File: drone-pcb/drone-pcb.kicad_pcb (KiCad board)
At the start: 2 copper layers, 50 x 50 mm, 13 parts, among them Q1 NMOS, Q2 NPN, Q3 NPN, U1 XIAO ESP32C3

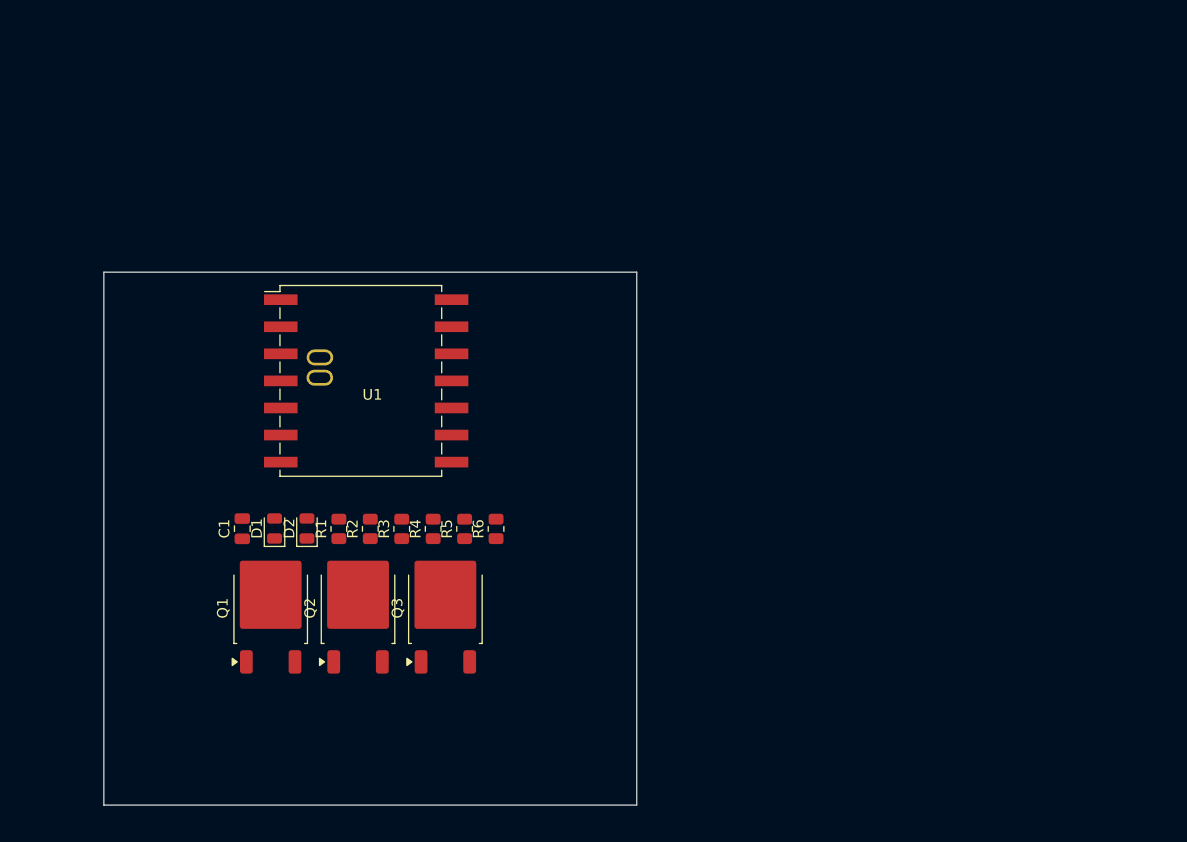
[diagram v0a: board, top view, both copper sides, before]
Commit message: draft pcb layout
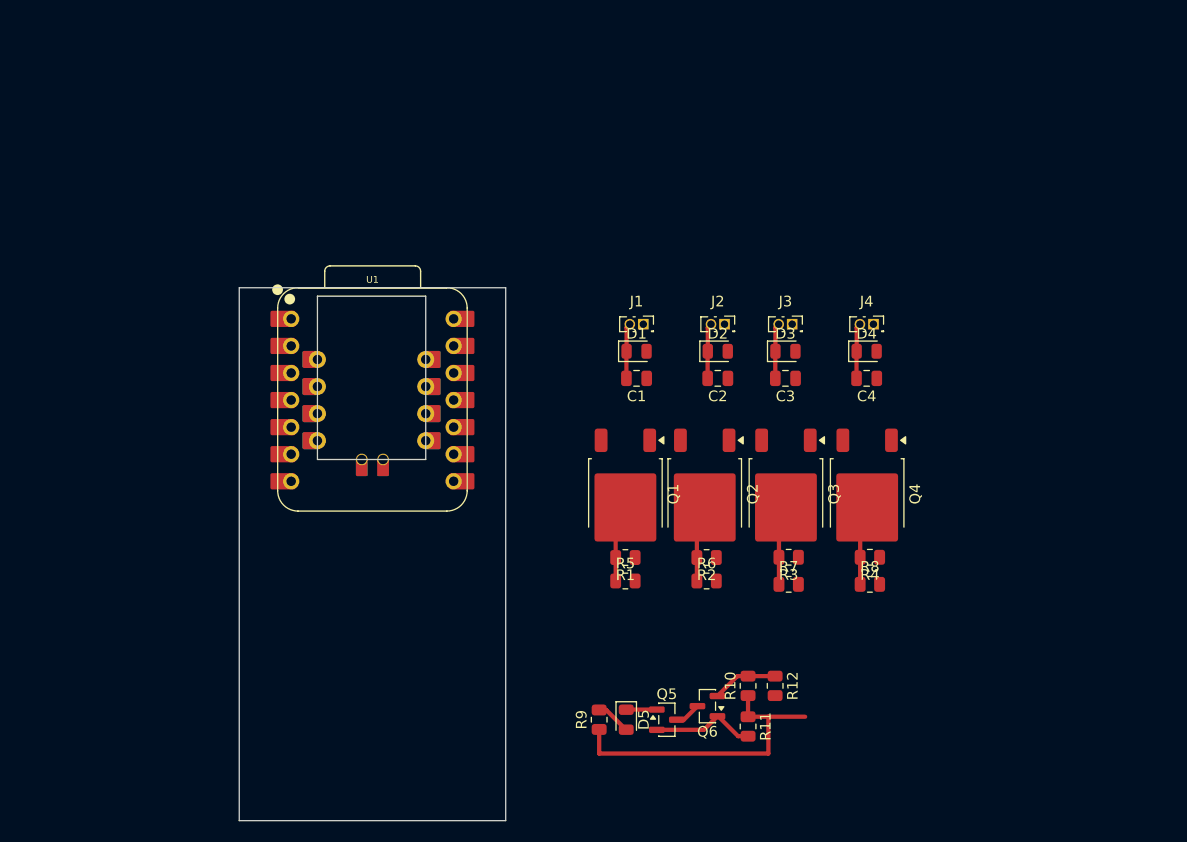
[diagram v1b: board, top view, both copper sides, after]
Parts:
- added C2: 0.1u, Capacitor_SMD:C_0805_2012Metric, F.Cu at (238.2, 48.2)
- added C3: 0.1u, Capacitor_SMD:C_0805_2012Metric, F.Cu at (244.6, 48.2)
- added C4: 0.1u, Capacitor_SMD:C_0805_2012Metric, F.Cu at (252.2, 48.2)
- added D3: 1N5819, Diode_SMD:D_0805_2012Metric, F.Cu at (244.6, 45.6)
- added D4: 1N5819, Diode_SMD:D_0805_2012Metric, F.Cu at (252.2, 45.6)
- added D5: LXZ1-PL02, Diode_SMD:D_0805_2012Metric, F.Cu at (229.6, 80.2)
- added J1: Conn_02x01, Connector_PinSocket_1.27mm:PinSocket_2x01_P1.27mm_Vertical, F.Cu at (231.2, 43.1)
- added J2: Conn_02x01, Connector_PinSocket_1.27mm:PinSocket_2x01_P1.27mm_Vertical, F.Cu at (238.8, 43.1)
- added J3: Conn_02x01, Connector_PinSocket_1.27mm:PinSocket_2x01_P1.27mm_Vertical, F.Cu at (245.2, 43.1)
- added J4: Conn_02x01, Connector_PinSocket_1.27mm:PinSocket_2x01_P1.27mm_Vertical, F.Cu at (252.8, 43.1)
- added Q4: NMOS, Package_TO_SOT_SMD:TO-252-2, F.Cu at (252.2, 59.0)
- added Q5: NPN, Package_TO_SOT_SMD:SOT-23, F.Cu at (233.4, 80.2)
- added Q6: NPN, Package_TO_SOT_SMD:SOT-23, F.Cu at (237.2, 78.9)
- added R10: 39k, Resistor_SMD:R_0805_2012Metric, F.Cu at (241.0, 77.0)
- added R11: 10k, Resistor_SMD:R_0805_2012Metric, F.Cu at (241.0, 80.8)
- added R12: 10k, Resistor_SMD:R_0805_2012Metric, F.Cu at (243.6, 77.0)
- added R7: 10k, Resistor_SMD:R_0805_2012Metric, F.Cu at (244.9, 67.5)
- added R8: 10k, Resistor_SMD:R_0805_2012Metric, F.Cu at (252.5, 67.5)
- added R9: 100, Resistor_SMD:R_0805_2012Metric, F.Cu at (227.1, 80.2)
- D2: value LXZ1-PL02 -> 1N5819
- Q2, Q3: value NPN -> NMOS
- R2, R4: value 10k -> 100
- R3: value 39k -> 100
- R6: value 100 -> 10k
- U1: value XIAO ESP32C3 -> XIAO-MG24-DIP; footprint libraries:xiao_esp32c3 -> libraries:XIAO-MG24-DIP
- moved D2 42.0 mm to (238.2, 45.6), turned to 0 degrees
- moved R4 41.1 mm to (252.5, 64.9), turned to 180 degrees
- moved C1 39.6 mm to (230.6, 48.2), turned to 180 degrees
- moved D1 37.8 mm to (230.6, 45.6), turned to 0 degrees
- moved R3 36.4 mm to (244.9, 64.9), turned to 180 degrees
- moved Q1 35.0 mm to (229.5, 59.0), turned to -90 degrees
- moved Q2 34.2 mm to (237.0, 59.0), turned to -90 degrees
- moved Q3 33.7 mm to (244.6, 59.0), turned to -90 degrees
- moved R2 31.7 mm to (237.2, 65.0), turned to 180 degrees
- moved R1 27.0 mm to (229.5, 65.0), turned to 180 degrees
- moved R6 20.4 mm to (237.2, 67.2), turned to 0 degrees
- moved R5 15.9 mm to (229.5, 67.2), turned to 0 degrees
- turned U1 to 90 degrees
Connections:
- net V_MOT+ renamed V_MOT1-
- net xiao_sense_G1 renamed Motor_1
- D2 pad 1: Net-(D2-K) -> V_BAT
- D2 pad 2: Net-(D2-A) -> V_MOT2-
- Q2 pad 1: Net-(Q2-C) -> V_MOT2-
- Q2 pad 2: Net-(Q2-B) -> Net-(Q2-G)
- Q3 pad 1: Net-(D2-K) -> V_MOT3-
- Q3 pad 2: Net-(Q2-C) -> Net-(Q3-G)
- R2 pad 1: Net-(Q1-G) -> Motor_2
- R2 pad 2: 0 -> Net-(Q2-G)
- R3 pad 1: V_BAT -> Motor_3
- R3 pad 2: Net-(Q2-B) -> Net-(Q3-G)
- R4 pad 1: Net-(Q2-B) -> Motor_4
- R4 pad 2: 0 -> Net-(Q4-G)
- R5 pad 1: V_BAT -> Net-(Q1-G)
- R5 pad 2: Net-(Q2-C) -> 0
- R6 pad 1: V_BAT -> Net-(Q2-G)
- R6 pad 2: Net-(D2-A) -> 0
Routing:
- net V_BAT: track 0.00 -> 49.8 mm
- net Net-(Q5-B): track 0.00 -> 9.89 mm
- net Net-(Q4-G): track 0.00 -> 7.87 mm
- net Net-(Q3-G): track 0.00 -> 7.87 mm
- net Net-(Q1-G): track 0.00 -> 7.81 mm
- net Net-(Q2-G): track 0.00 -> 7.64 mm
- net Net-(Q6-B): track 0.00 -> 6.19 mm
- net Net-(D5-A): track 0.00 -> 3.34 mm
- net Net-(D5-K): track 0.00 -> 2.88 mm
- net 0: track 0.00 -> 2.46 mm
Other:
- board size 50 x 50 mm -> 25 x 50 mm

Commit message: apdejt
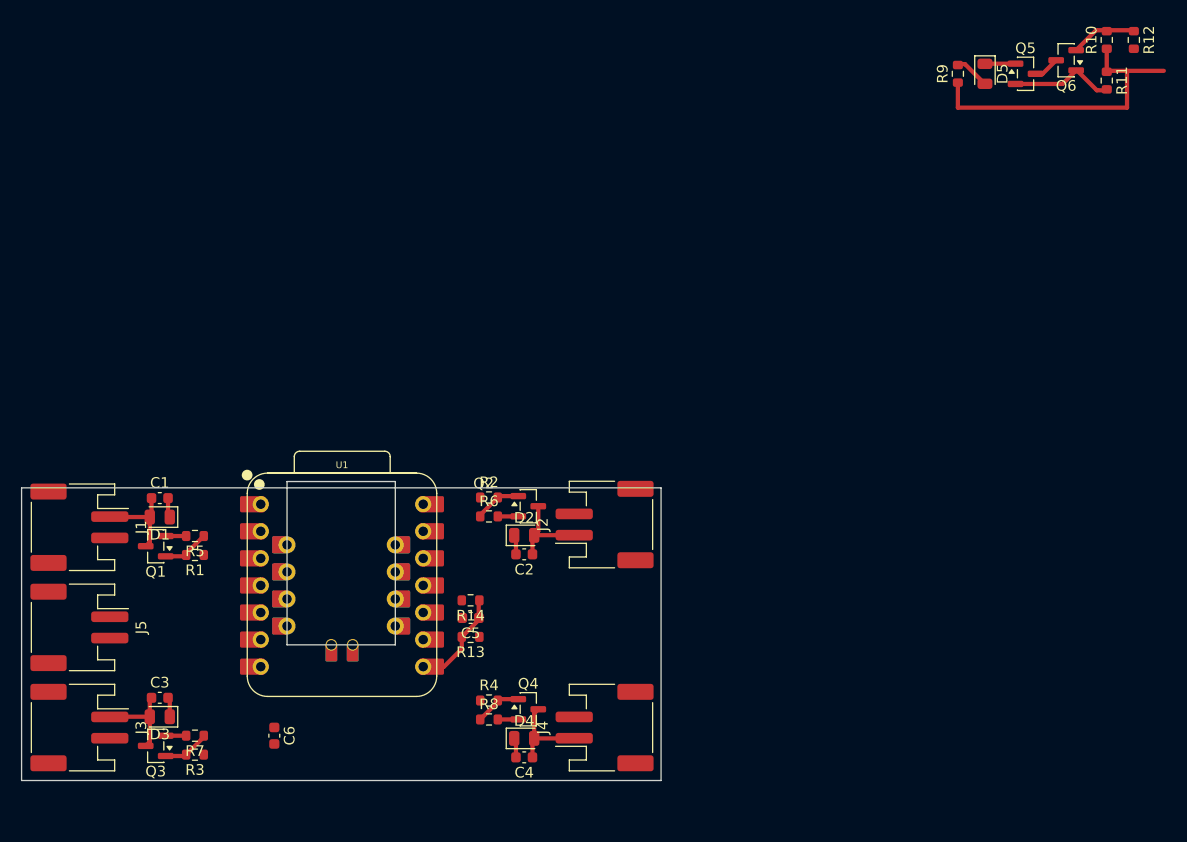
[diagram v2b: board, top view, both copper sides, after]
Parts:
- added C5: 0.1u, Capacitor_SMD:C_0603_1608Metric, F.Cu at (215.0, 70.6)
- added C6: 470u, Capacitor_SMD:C_0603_1608Metric, F.Cu at (196.6, 81.7)
- added J5: Conn_02x01, jst:JST_PH_S2B-PH-SM4-TB_1x02-1MP_P2.00mm_Horizontal_footprint, F.Cu at (178.3, 71.5)
- added R13: 470k, Resistor_SMD:R_0603_1608Metric, F.Cu at (215.0, 72.4)
- added R14: 470k, Resistor_SMD:R_0603_1608Metric, F.Cu at (215.0, 69.0)
- C1, C2, C3, C4: footprint Capacitor_SMD:C_0805_2012Metric -> Capacitor_SMD:C_0603_1608Metric
- J1, J2, J3, J4: footprint Connector_PinSocket_1.27mm:PinSocket_2x01_P1.27mm_Vertical -> jst:JST_PH_S2B-PH-SM4-TB_1x02-1MP_P2.00mm_Horizontal_footprint
- Q1, Q2, Q3, Q4: footprint Package_TO_SOT_SMD:TO-252-2 -> Package_TO_SOT_SMD:SOT-23
- R1, R10, R11, R12, R2, R3, R4, R5, R6, R7, R8, R9: footprint Resistor_SMD:R_0805_2012Metric -> Resistor_SMD:R_0603_1608Metric
- moved J3 76.8 mm to (178.3, 80.9), turned to -90 degrees
- moved R10 69.3 mm to (274.7, 16.4)
- moved R11 69.3 mm to (274.7, 20.2)
- moved R12 69.3 mm to (277.2, 16.4)
- moved R9 69.3 mm to (260.7, 19.6)
- moved Q6 69.3 mm to (270.9, 18.3)
- moved D5 69.3 mm to (263.3, 19.6)
- moved Q5 69.3 mm to (267.1, 19.6)
- moved D3 68.0 mm to (185.8, 79.9), turned to 180 degrees
- moved C3 65.9 mm to (185.8, 78.1), turned to 0 degrees
- moved Q3 63.7 mm to (185.5, 82.6), turned to 180 degrees
- moved R3 58.7 mm to (189.2, 83.5)
- moved R7 57.5 mm to (189.2, 81.7), turned to 180 degrees
- moved J1 56.2 mm to (178.3, 62.1), turned to -90 degrees
- moved D4 48.5 mm to (220.0, 81.9)
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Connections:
- Q1 pad 1: V_MOT1- -> Net-(Q1-G)
- Q1 pad 2: Net-(Q1-G) -> GND
- Q1 pad 3: 0 -> V_MOT1-
- Q2 pad 1: V_MOT2- -> Net-(Q2-D)
- Q2 pad 2: Net-(Q2-G) -> GND
- Q2 pad 3: 0 -> V_MOT2-
- Q3 pad 1: V_MOT3- -> Net-(Q3-D)
- Q3 pad 2: Net-(Q3-G) -> GND
- Q3 pad 3: 0 -> V_MOT3-
- Q4 pad 1: V_MOT4- -> Net-(Q4-D)
- Q4 pad 2: Net-(Q4-G) -> GND
- Q4 pad 3: 0 -> V_MOT4-
- R2 pad 2: Net-(Q2-G) -> Net-(Q2-D)
- R3 pad 2: Net-(Q3-G) -> Net-(Q3-D)
- R4 pad 2: Net-(Q4-G) -> Net-(Q4-D)
- R5 pad 2: 0 -> GND
- R6 pad 1: Net-(Q2-G) -> Net-(Q2-D)
- R6 pad 2: 0 -> GND
- R7 pad 1: Net-(Q3-G) -> Net-(Q3-D)
- R7 pad 2: 0 -> GND
- R8 pad 1: Net-(Q4-G) -> Net-(Q4-D)
- R8 pad 2: 0 -> GND
- U1 pad 1: unconnected-(U1-PC00_A0_D0-Pad1) -> Motor_1
- U1 pad 10: unconnected-(U1-PA04_A9_D9_MISO-Pad10) -> Motor_4
- U1 pad 11: unconnected-(U1-PA05_A10_D10_MOSI-Pad11) -> Motor_2
- U1 pad 13: unconnected-(U1-GND-Pad13) -> GND
- U1 pad 2: unconnected-(U1-PC01_A1_D1-Pad2) -> Motor_3
- U1 pad 8: unconnected-(U1-PC07_A7_D7_RX-Pad8) -> Net-(U1-PC07_A7_D7_RX)
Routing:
- net V_BAT: track 49.8 -> 36.3 mm
- net Net-(U1-PC07_A7_D7_RX): track 0.00 -> 8.78 mm
- net V_MOT1-: track 0.00 -> 8.51 mm
- net V_MOT4-: track 0.00 -> 8.50 mm
- net V_MOT2-: track 0.00 -> 8.50 mm
- net V_MOT3-: track 0.00 -> 8.50 mm
- net Net-(Q4-G): track 7.87 -> 0.00 mm
- net Net-(Q3-G): track 7.87 -> 0.00 mm
- net GND: track 0.00 -> 7.69 mm
- net Net-(Q2-G): track 7.64 -> 0.00 mm
- net Net-(Q2-D): track 0.00 -> 4.43 mm
- net Net-(Q3-D): track 0.00 -> 4.43 mm
- net Net-(Q4-D): track 0.00 -> 4.36 mm
- net Net-(Q1-G): track 7.81 -> 4.43 mm
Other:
- board size 25 x 50 mm -> 60 x 27.5 mm
